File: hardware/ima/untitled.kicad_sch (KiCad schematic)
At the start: 9 parts, among them J2 61201021621, U3 NCP711BMT330TBG, U4 NCP711BMT330TBG

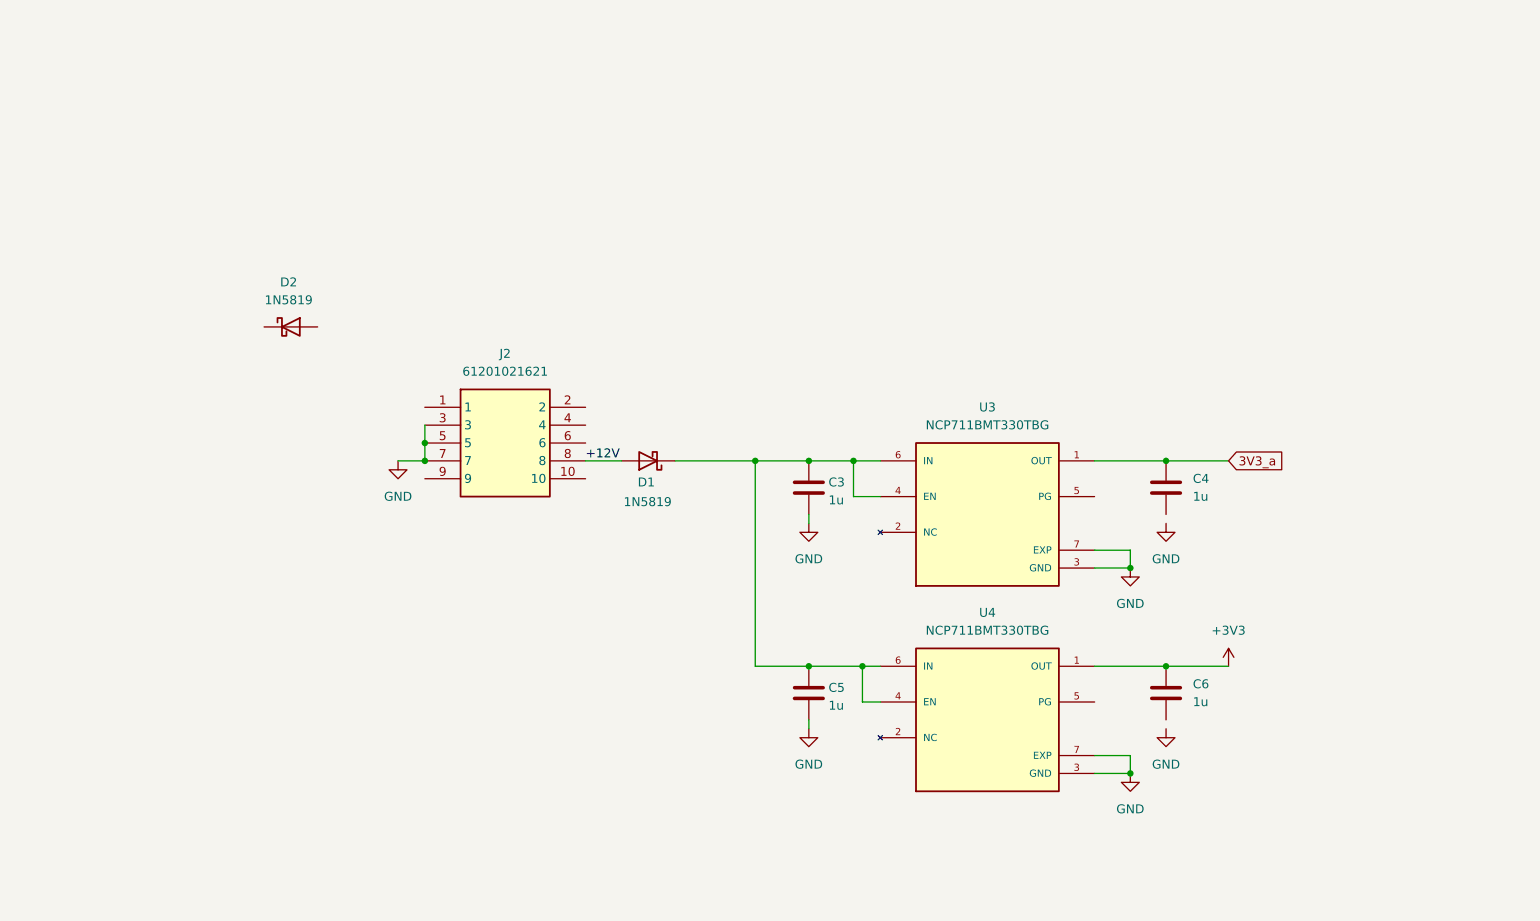
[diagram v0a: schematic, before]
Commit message: update docs
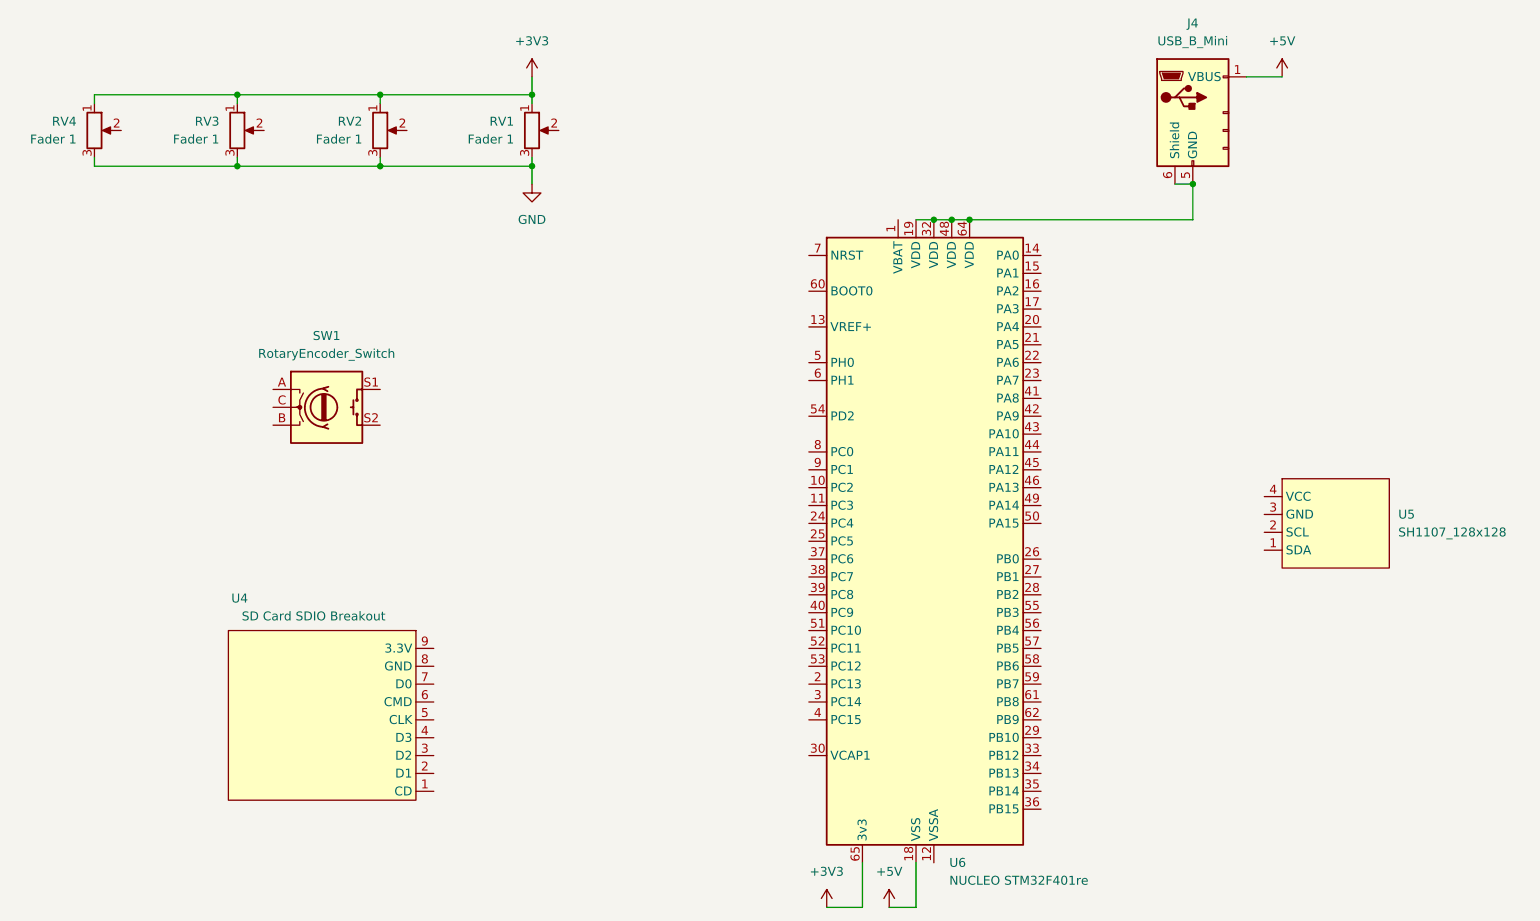
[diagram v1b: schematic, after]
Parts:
- removed C3, C4, C5, C6: 1u, symbol Device:C
- removed D1, D2: 1N5819, Diode_THT:D_DO-41_SOD81_P10.16mm_Horizontal, symbol Diode:1N5819
- removed J2: 61201021621, SHDR10W64P254_2X5_2036X885X925P, symbol 61201021621:61201021621
- removed U3, U4: NCP711BMT330TBG, NCP711BMT330TBG:SON65P200X200X80-7N, symbol NCP711BMT330TBG:NCP711BMT330TBG
- added J4: USB_B_Mini, symbol Connector:USB_B_Mini
- added RV1, RV2, RV3, RV4: Fader 1, symbol Device:R_Potentiometer
- added SW1: RotaryEncoder_Switch, symbol Device:RotaryEncoder_Switch
- added U4: SD Card SDIO Breakout, symbol New_Library:Waveshare_SD_Card_Breakout
- added U5: SH1107_128x128, symbol New_Library:128x128Display
- added U6: NUCLEO STM32F401re, Package_QFP:LQFP-64_10x10mm_P0.5mm, symbol MCU_ST_STM32F4:STM32F401RETx
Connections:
- net +3V3: now also RV1.1, RV2.1, RV3.1, RV4.1, U6.65 (3v3)
- net GND: now also RV1.3, RV2.3, RV3.3, RV4.3
- new net: J4.5 (GND), J4.6 (Shield), U6.19 (VDD), U6.32 (VDD), U6.48 (VDD), U6.64 (VDD)
- new net +5V: J4.1 (VBUS), U6.18 (VSS), U6.31 (VSS), U6.47 (VSS), U6.63 (VSS)
